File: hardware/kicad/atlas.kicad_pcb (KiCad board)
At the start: 4 copper layers, 38.4 x 82.2 mm, 121 parts, among them J1 U262-161N-4BVC11, J2 +LIPO, J3 -LIPO, J4 HC-FPC-05-09-24RLTAG, Q1 DMG1012UW, Q4 PMV32UP, Q5 DMG1012UW, Q6 AO3407A, Q7 SI1308EDL, Q8 PMV32UP, Q9 DMG1012UW, SW1 B3U-3000P, SW2 B3U-3000P, SW3 B3U-3000P, U1 ESP32-C6FH4, U10 L86-M33, U2 USBLC6-2P6, U3 MCP73831T-2ACI/OT, U4 AEM10941, U6 XC6220, U7 BME688, Y1 CM315D32768DZFT, Y2 R940000171

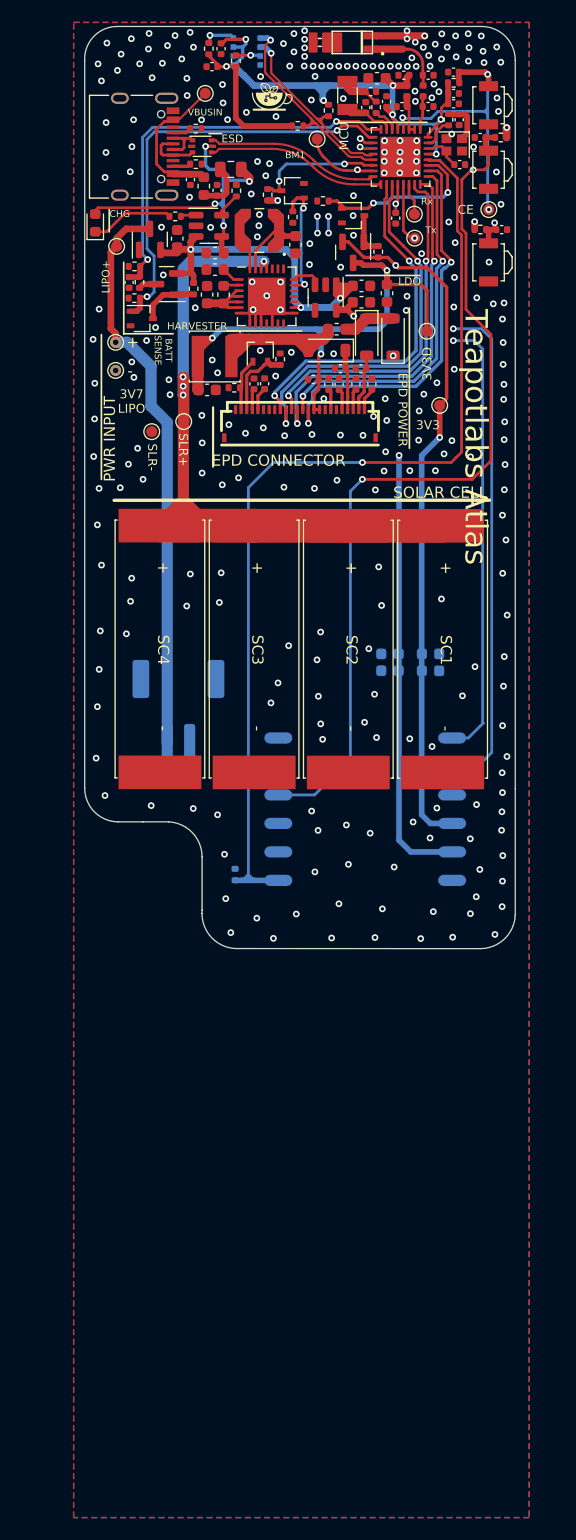
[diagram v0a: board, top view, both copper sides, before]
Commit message: added led symbols and placements on pcb.
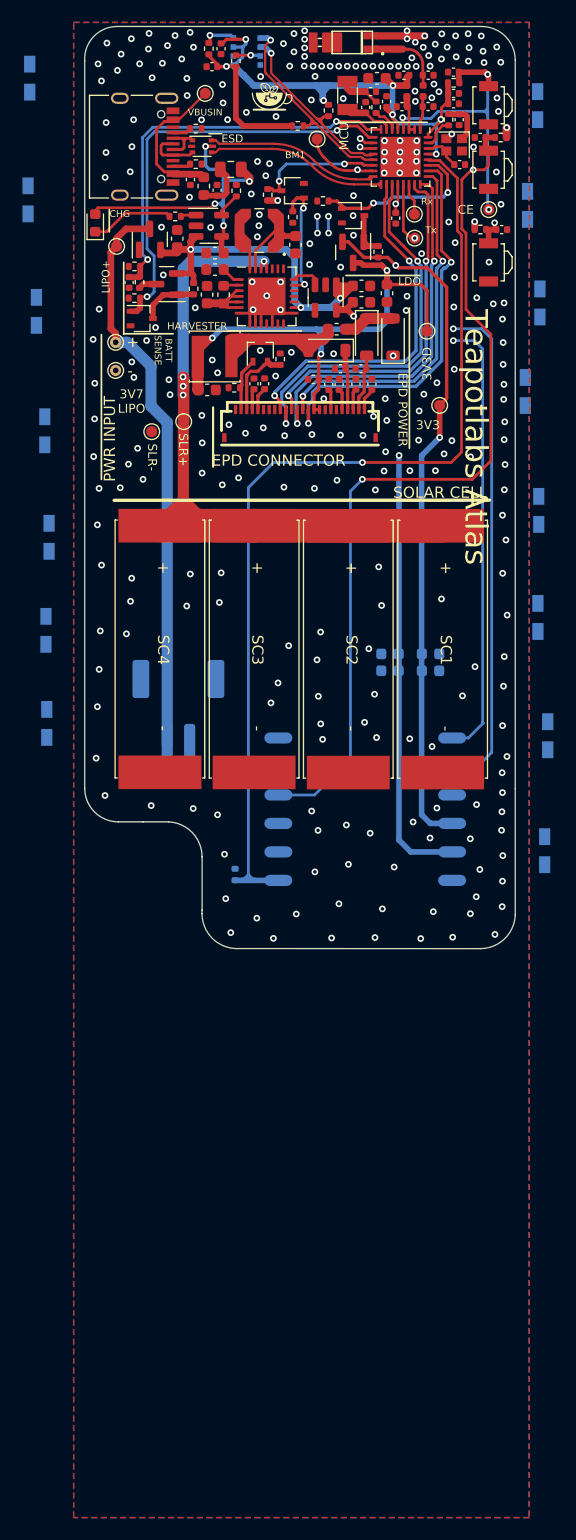
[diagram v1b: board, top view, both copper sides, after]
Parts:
- added LED**: LTSTS220KGKT, ltst-220:LTSTS220KGKT, B.Cu at (85.6, 37.5)
- added LED**: LTSTS220KGKT, ltst-220:LTSTS220KGKT, B.Cu at (130.0, 48.9)
- added LED**: LTSTS220KGKT, ltst-220:LTSTS220KGKT, B.Cu at (131.0, 76.1)
- added LED**: LTSTS220KGKT, ltst-220:LTSTS220KGKT, B.Cu at (131.8, 96.2)
- added LED**: LTSTS220KGKT, ltst-220:LTSTS220KGKT, B.Cu at (87.3, 78.5)
- added LED**: LTSTS220KGKT, ltst-220:LTSTS220KGKT, B.Cu at (131.5, 106.5)
- added LED**: LTSTS220KGKT, ltst-220:LTSTS220KGKT, B.Cu at (130.9, 40.0)
- added LED**: LTSTS220KGKT, ltst-220:LTSTS220KGKT, B.Cu at (87.1, 95.1)
- added LED**: LTSTS220KGKT, ltst-220:LTSTS220KGKT, B.Cu at (86.9, 69.0)
- added LED**: LTSTS220KGKT, ltst-220:LTSTS220KGKT, B.Cu at (131.1, 57.6)
- added LED**: LTSTS220KGKT, ltst-220:LTSTS220KGKT, B.Cu at (86.2, 58.4)
- added LED**: LTSTS220KGKT, ltst-220:LTSTS220KGKT, B.Cu at (87.0, 86.8)
- added LED**: LTSTS220KGKT, ltst-220:LTSTS220KGKT, B.Cu at (85.4, 48.4)
- added LED**: LTSTS220KGKT, ltst-220:LTSTS220KGKT, B.Cu at (129.8, 65.5)
- added LED**: LTSTS220KGKT, ltst-220:LTSTS220KGKT, B.Cu at (130.9, 85.7)

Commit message: Revert "added led symbols and placements on pcb."
This reverts commit 775bc6ae91366f689438663b29cde4e2220ca0a7.
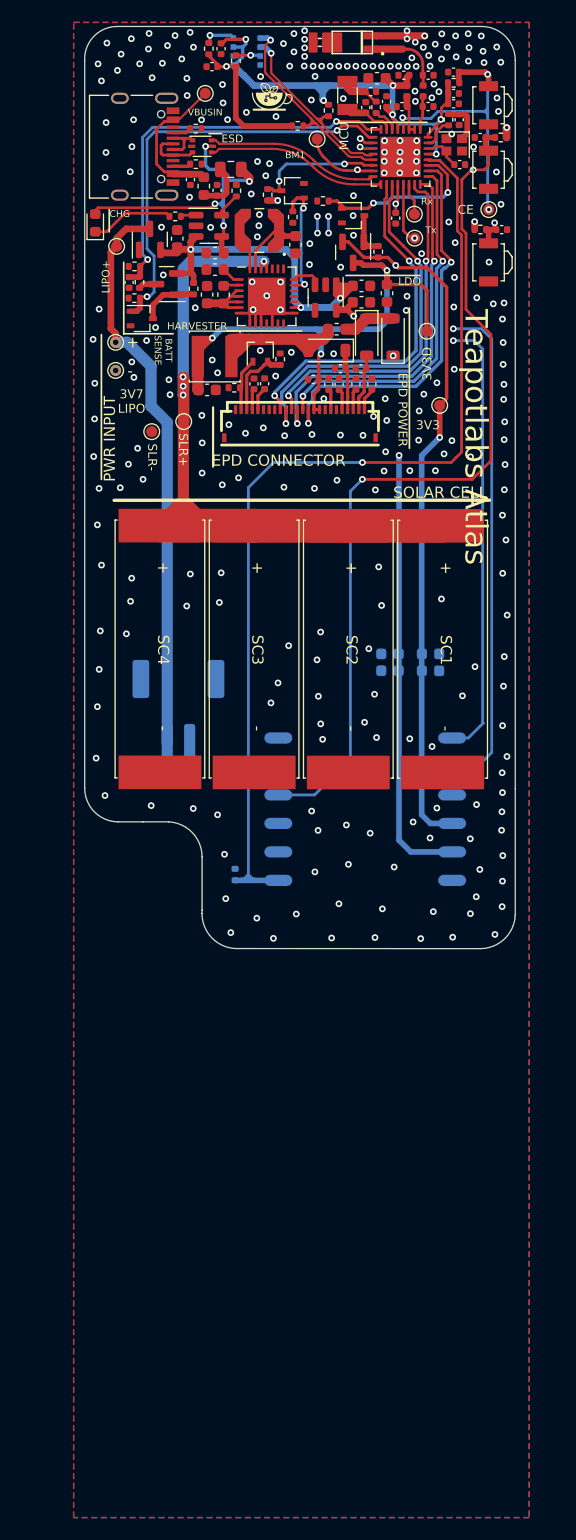
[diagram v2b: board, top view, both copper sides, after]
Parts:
- removed LED** (x15): LTSTS220KGKT, ltst-220:LTSTS220KGKT
